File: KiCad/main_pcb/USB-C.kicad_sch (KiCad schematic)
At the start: 9 parts, among them J2 USB-C, U10 JSMSEMI AMS1117-3.3V, U8 CH340C

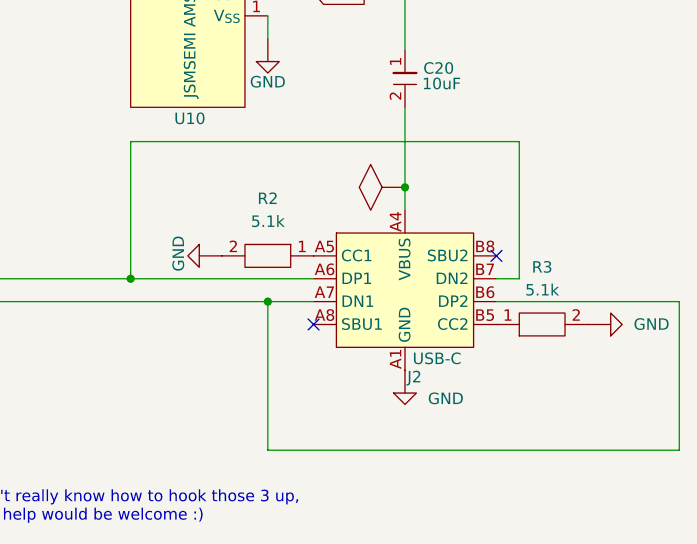
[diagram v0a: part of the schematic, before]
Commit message: feat(KiCad): Continues work on circuit
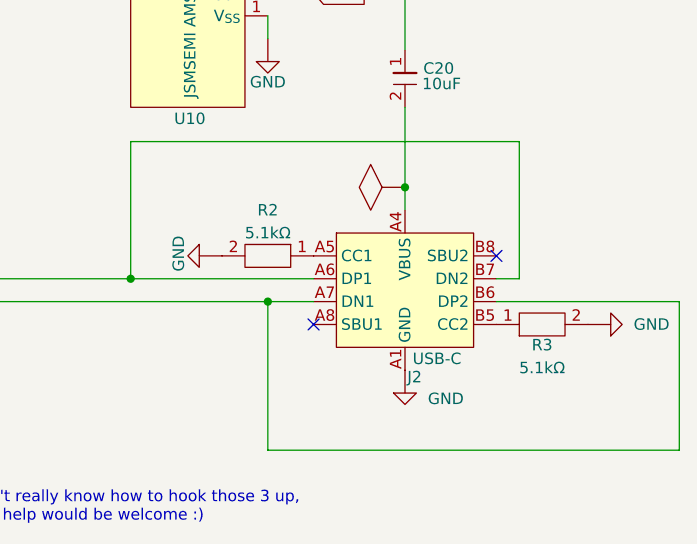
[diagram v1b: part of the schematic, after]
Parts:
- R2, R3: value 5.1k -> 5.1kΩ
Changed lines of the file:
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@@
 		(in_pos_files yes)
 		(dnp no)
-		(fields_autoplaced yes)
 		(property "Reference" "R3"
-			(at 184.15 104.14 90)
-			(show_name no)
-			(do_not_autoplace no)
-			(effects
-				(font
-					(size 1.27 1.27)
-				)
-			)
-		)
-		(property "Value" "5.1k"
-			(at 184.15 106.68 90)
+			(at 184.15 112.776 90)
+			(show_name no)
+			(do_not_autoplace no)
+			(effects
+				(font
+					(size 1.27 1.27)
+				)
+			)
+		)
+		(property "Value" "5.1kΩ"
+			(at 184.15 115.316 90)
 			(show_name no)
 			(do_not_autoplace no)
@@
 		(in_pos_files yes)
 		(dnp no)
-		(fields_autoplaced yes)
 		(property "Reference" "R2"
-			(at 153.67 96.52 90)
-			(show_name no)
-			(do_not_autoplace no)
-			(effects
-				(font
-					(size 1.27 1.27)
-				)
-			)
-		)
-		(property "Value" "5.1k"
-			(at 153.67 99.06 90)
-			(show_name no)
-			(do_not_autoplace no)
+			(at 153.67 97.79 90)
+			(show_name no)
+			(do_not_autoplace no)
+			(effects
+				(font
+					(size 1.27 1.27)
+				)
+			)
+		)
+		(property "Value" "5.1kΩ"
+			(at 153.67 100.33 90)
+			(show_name no)
+			(do_not_autoplace no)
